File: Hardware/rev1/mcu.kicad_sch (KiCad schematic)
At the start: 18 parts, among them Q1 AO3400A, SW1 SW_Push, U0 STM32F103C8Tx, Y1 16MHz

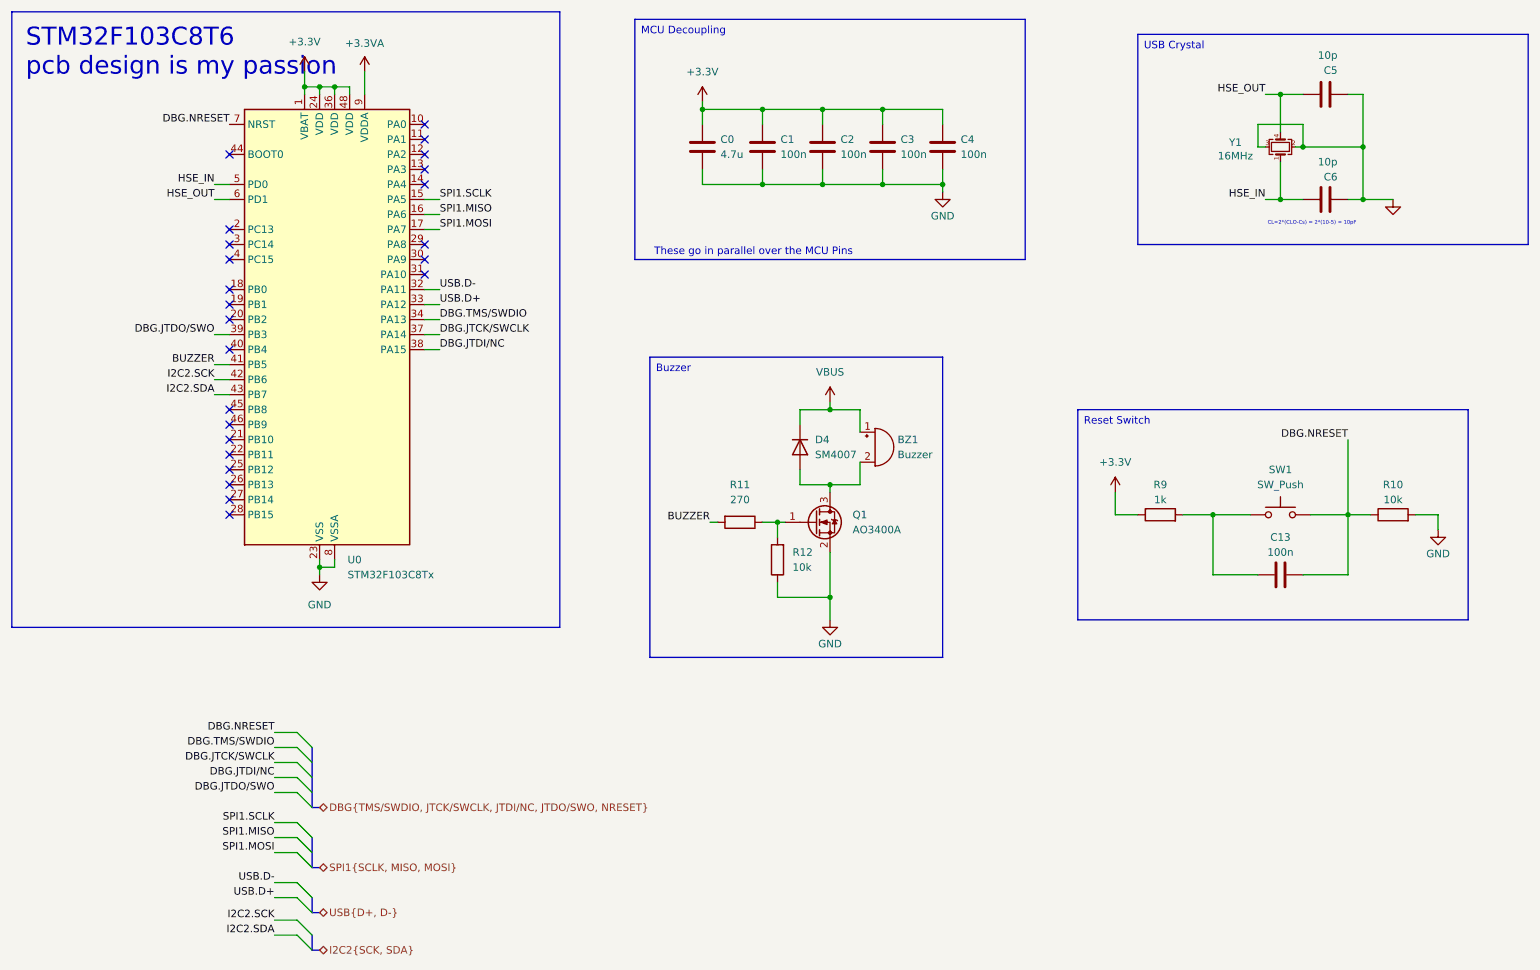
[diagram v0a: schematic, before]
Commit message: Revert "Merge remote-tracking branch 'origin/dev'"
This reverts commit 9d6b38d1428df59ab2602e839e1db75647d3fbc2, reversing
changes made to aa461fd2fa90bcdcb689545e3dbed326723346fe.
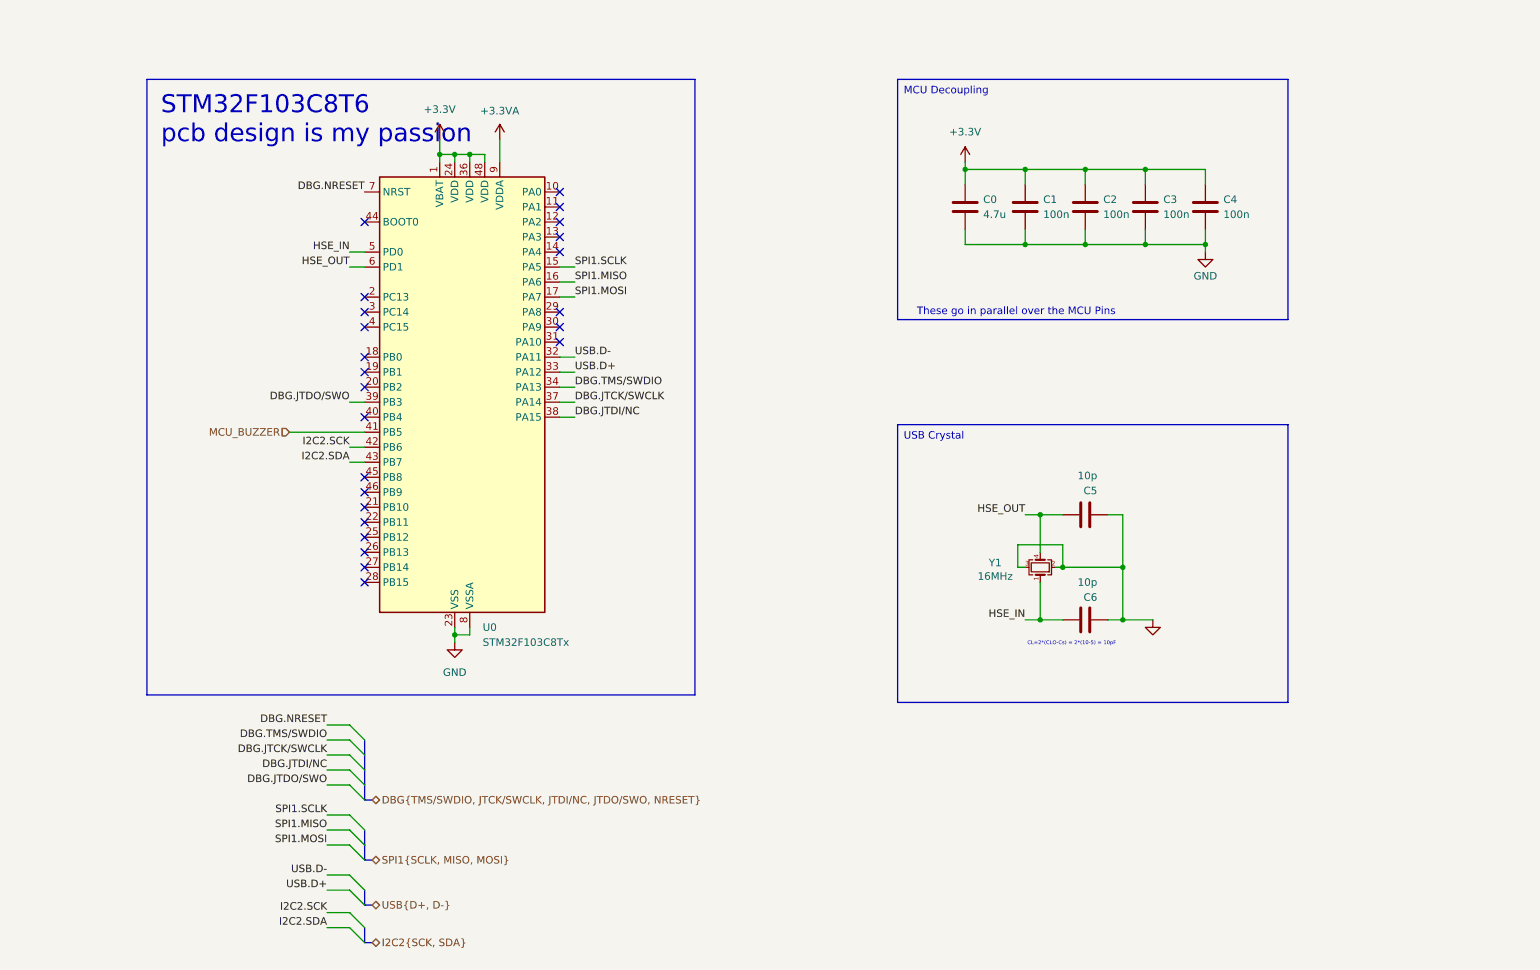
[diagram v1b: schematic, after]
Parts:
- removed BZ1: Buzzer, Buzzer_Beeper:MagneticBuzzer_Kingstate_KCG0601, symbol Device:Buzzer
- removed C13: 100n, Capacitor_SMD:C_0402_1005Metric, symbol Device:C
- removed D4: SM4007, Diode_SMD:D_SOD-123F, symbol Diode:SM4007
- removed Q1: AO3400A, Package_TO_SOT_SMD:SOT-23, symbol Transistor_FET:AO3400A
- removed R10, R12: 10k, Resistor_SMD:R_0603_1608Metric, symbol Device:R
- removed R11: 270, Resistor_SMD:R_0603_1608Metric, symbol Device:R
- removed R9: 1k, Resistor_SMD:R_0603_1608Metric, symbol Device:R
- removed SW1: SW_Push, Button_Switch_SMD:SW_Push_1P1T_XKB_TS-1187A, symbol Switch:SW_Push
- C0: footprint Buzzer_Beeper:MagneticBuzzer_Kingstate_KCG0601 -> (none)
- C1, C2, C3, C4: footprint Capacitor_SMD:C_0402_1005Metric -> (none)
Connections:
- net BUZZER renamed MCU_BUZZER
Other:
- moved on the sheet: C0, C1, C2, C3, C4, C5, C6, U0, Y1
